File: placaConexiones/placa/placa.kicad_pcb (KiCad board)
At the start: 2 copper layers, 38.1 x 51.2 mm, 12 parts, among them J1 Conn_01x05, J2 Conn_01x05, J3 Conn_01x06, J4 Conn_01x09

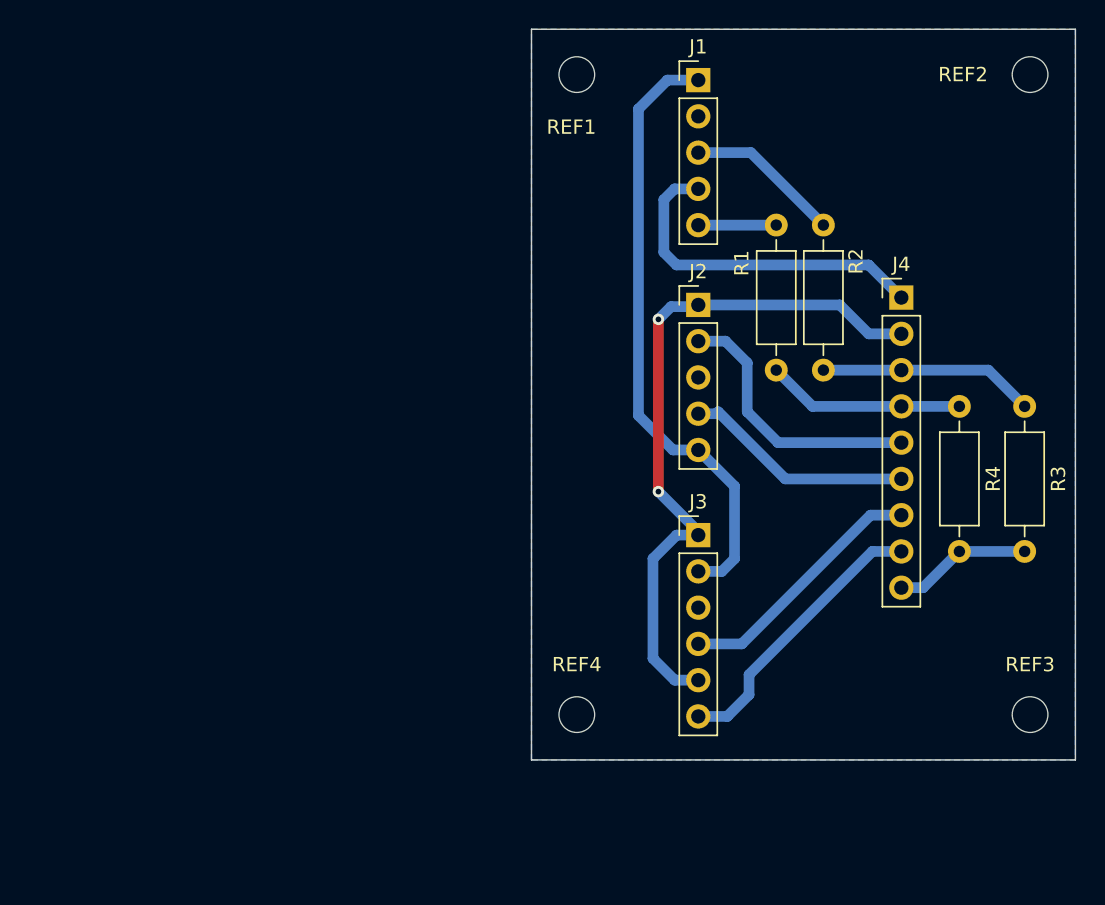
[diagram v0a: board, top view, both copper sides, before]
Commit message: Cambios modelos y diseños
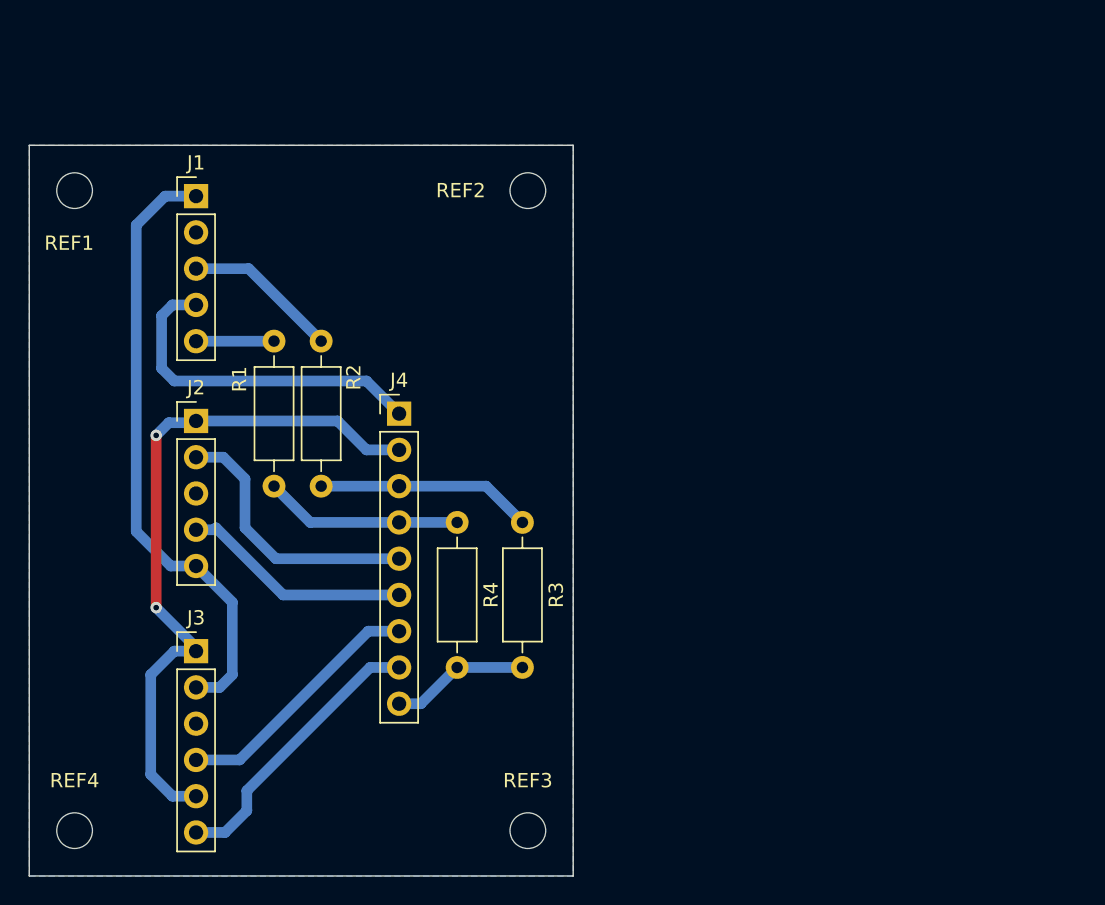
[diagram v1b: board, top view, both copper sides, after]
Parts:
- moved J1 36.1 mm to (136.5, 62.5)
- moved J2 36.1 mm to (136.5, 78.2)
- moved J3 36.1 mm to (136.5, 94.4)
- moved J4 36.1 mm to (150.7, 77.7)
- moved R1 36.1 mm to (142.0, 72.6)
- moved R2 36.1 mm to (145.3, 72.6)
- moved R3 36.1 mm to (159.4, 85.3)
- moved R4 36.1 mm to (154.8, 85.3)
- moved REF1 36.1 mm to (128.0, 62.1)
- moved REF2 36.1 mm to (159.8, 62.1)
- moved REF3 36.1 mm to (159.8, 106.9)
- moved REF4 36.1 mm to (128.0, 106.9)
